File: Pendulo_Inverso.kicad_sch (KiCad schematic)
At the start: 6 parts, among them IC2 TB6612FNG, U1 LM7805_TO220, U2 ESP32-DEVKITC, U4 MPU-6050-A

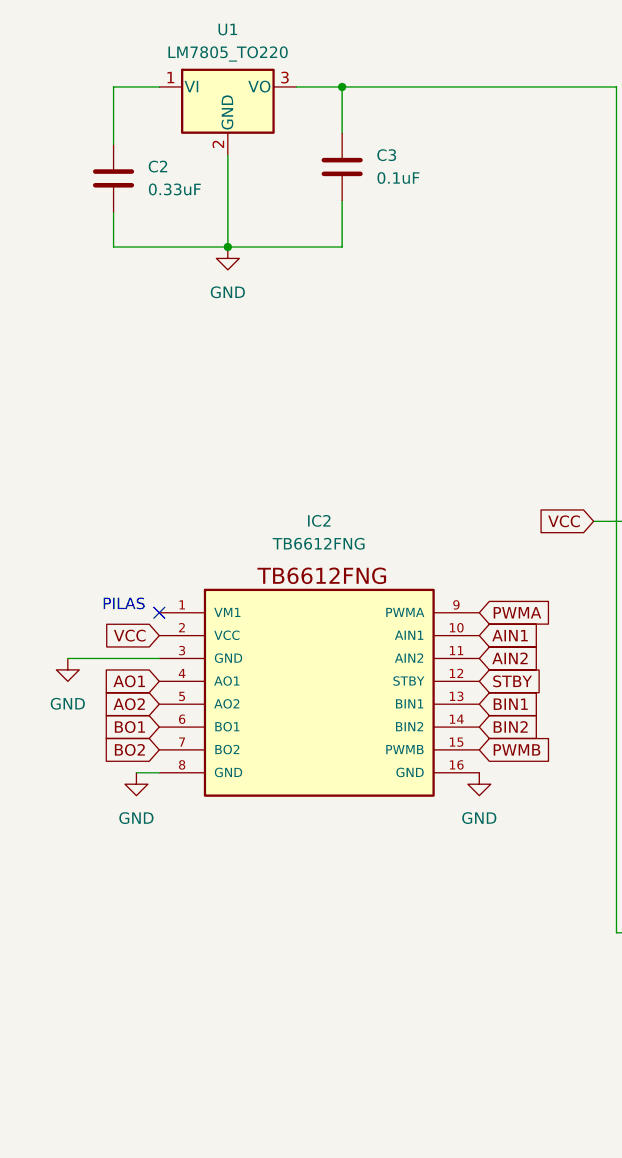
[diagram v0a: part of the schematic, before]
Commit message: modified:   Pendulo_Inverso.dsn 	modified:   Pendulo_Inverso.kicad_pcb 	modified:   Pendulo_Inverso.kicad_prl 	modified:   Pendulo_Inverso.kicad_sch 	modified:   Pendulo_Inverso.rules 	modified:   Pendulo_Inverso.ses 	modified:   fp-info-cache
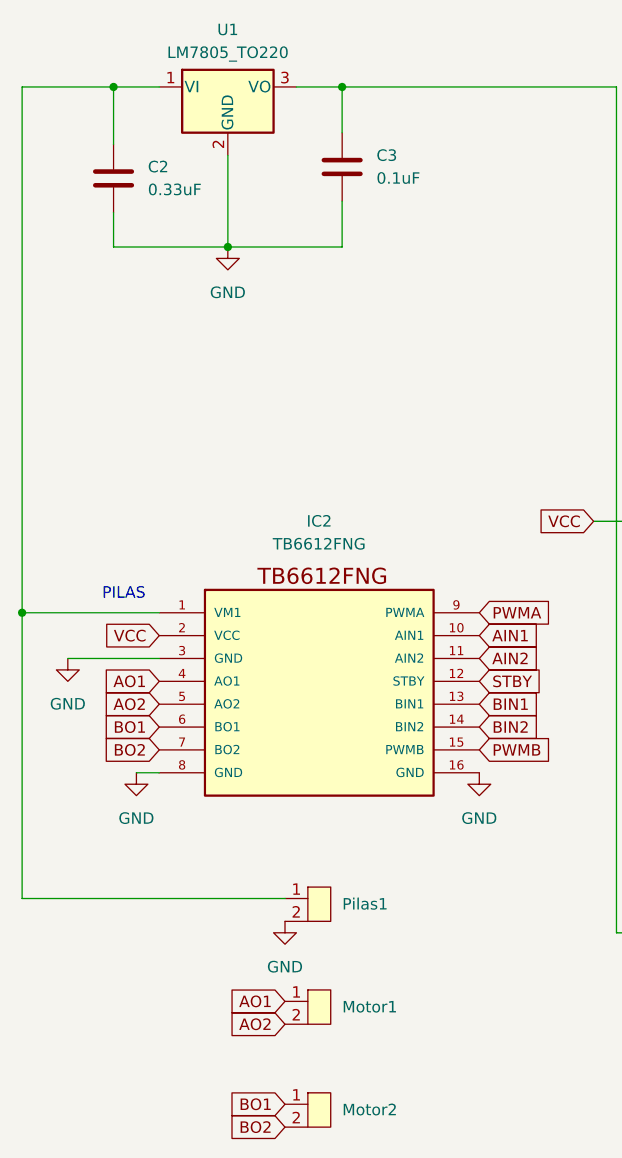
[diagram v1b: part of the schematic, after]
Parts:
- added Motor1, Motor2, Pilas1: ~, Mi_Libreria2:Conector_doble, symbol Mi_Libreria:Conector_doble
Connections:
- net AO1: now also Motor1.1
- net AO2: now also Motor1.2
- net BO1: now also Motor2.1
- net BO2: now also Motor2.2
- net GND: now also Pilas1.2
- net at C2.1, U1.1 (VI): now also IC2.1 (VM1), Pilas1.1
- no-connect marks 31 -> 30
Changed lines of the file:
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@@
   (junction (at 132.08 88.9) (diameter 0) (color 0 0 0 0)
   )
+  (junction (at 60.96 99.06) (diameter 0) (color 0 0 0 0)
+  )
   (junction (at 83.82 58.42) (diameter 0) (color 0 0 0 0)
+  )
+  (junction (at 71.12 40.64) (diameter 0) (color 0 0 0 0)
   )
   (junction (at 96.52 40.64) (diameter 0) (color 0 0 0 0)
@@
   (no_connect (at 132.08 93.98))
   (no_connect (at 132.08 101.6))
-  (no_connect (at 76.2 99.06))
   (no_connect (at 132.08 104.14))
   (no_connect (at 172.72 96.52))
@@
     (stroke (width 0) (type default))
   )
+  (wire (pts (xy 60.96 130.81) (xy 90.17 130.81))
+    (stroke (width 0) (type default))
+  )
   (wire (pts (xy 96.52 40.64) (xy 127 40.64))
     (stroke (width 0) (type default))
@@
     (stroke (width 0) (type default))
   )
+  (wire (pts (xy 71.12 40.64) (xy 60.96 40.64))
+    (stroke (width 0) (type default))
+  )
   (wire (pts (xy 172.72 104.14) (xy 177.8 104.14))
     (stroke (width 0) (type default))
@@
     (stroke (width 0) (type default))
   )
+  (wire (pts (xy 60.96 40.64) (xy 60.96 99.06))
+    (stroke (width 0) (type default))
+  )
   (wire (pts (xy 180.34 101.6) (xy 180.34 104.14))
     (stroke (width 0) (type default))
   )
+  (wire (pts (xy 60.96 99.06) (xy 60.96 130.81))
+    (stroke (width 0) (type default))
+  )
   (wire (pts (xy 71.12 54.61) (xy 71.12 58.42))
     (stroke (width 0) (type default))
@@
     (stroke (width 0) (type default))
   )
+  (wire (pts (xy 76.2 99.06) (xy 60.96 99.06))
+    (stroke (width 0) (type default))
+  )
   (wire (pts (xy 127 134.62) (xy 132.08 134.62))
     (stroke (width 0) (type default))
   )
-  (text "PILAS" (at 69.85 99.06 0)
+  (text "PILAS" (at 69.85 97.79 0)
     (effects (font (size 1.27 1.27)) (justify left bottom))
   )
@@
     )
   )
+  (global_label "AO1" (shape input) (at 90.17 142.24 180) (fields_autoplaced)
+    (effects (font (size 1.27 1.27)) (justify right))
+    (property "Intersheetrefs" "${INTERSHEET_REFS}" (at 83.5562 142.24 0)
+      (effects (font (size 1.27 1.27)) (justify right) hide)
+    )
+  )
   (global_label "BO2" (shape input) (at 76.2 114.3 180) (fields_autoplaced)
     (effects (font (size 1.27 1.27)) (justify right))
@@
     )
   )
+  (global_label "BO2" (shape input) (at 90.17 156.21 180) (fields_autoplaced)
+    (effects (font (size 1.27 1.27)) (justify right))
+    (property "Intersheetrefs" "${INTERSHEET_REFS}" (at 83.3748 156.21 0)
+      (effects (font (size 1.27 1.27)) (justify right) hide)
+    )
+  )
+  (global_label "BO1" (shape input) (at 90.17 153.67 180) (fields_autoplaced)
+    (effects (font (size 1.27 1.27)) (justify right))
+    (property "Intersheetrefs" "${INTERSHEET_REFS}" (at 83.3748 153.67 0)
+      (effects (font (size 1.27 1.27)) (justify right) hide)
+    )
+  )
   (global_label "BIN2" (shape input) (at 111.76 111.76 0) (fields_autoplaced)
     (effects (font (size 1.27 1.27)) (justify left))
@@
     )
   )
+  (global_label "AO2" (shape input) (at 90.17 144.78 180) (fields_autoplaced)
+    (effects (font (size 1.27 1.27)) (justify right))
+    (property "Intersheetrefs" "${INTERSHEET_REFS}" (at 83.5562 144.78 0)
+      (effects (font (size 1.27 1.27)) (justify right) hide)
+    )
+  )
   (global_label "PWMB" (shape input) (at 111.76 114.3 0) (fields_autoplaced)
     (effects (font (size 1.27 1.27)) (justify left))
@@
         (path "/efb3785d-97dd-4c84-bd5b-f8cfd60b2cf2"
           (reference "#PWR04") (unit 1)
+        )
+      )
+    )
+  )
+  (symbol (lib_id "power:GND") (at 90.17 133.35 0) (unit 1)
+    (in_bom yes) (on_board yes) (dnp no) (fields_autoplaced)
+    (property "Reference" "#PWR09" (at 90.17 139.7 0)
+      (effects (font (size 1.27 1.27)) hide)
+    )
+    (property "Value" "GND" (at 90.17 138.43 0)
+      (effects (font (size 1.27 1.27)))
+    )
+    (property "Footprint" "" (at 90.17 133.35 0)
+      (effects (font (size 1.27 1.27)) hide)
+    )
+    (property "Datasheet" "" (at 90.17 133.35 0)
+      (effects (font (size 1.27 1.27)) hide)
+    )
+    (pin "1")
+    (instances
+      (project "Pendulo_Inverso"
+        (path "/efb3785d-97dd-4c84-bd5b-f8cfd60b2cf2"
+          (reference "#PWR09") (unit 1)
+        )
+      )
+    )
+  )
+  (symbol (lib_id "Mi_Libreria:Conector_doble") (at 90.17 153.67 0) (unit 1)
+    (in_bom yes) (on_board yes) (dnp no) (fields_autoplaced)
+    (property "Reference" "Motor2" (at 96.52 154.305 0)
+      (effects (font (size 1.27 1.27)) (justify left))
+    )
+    (property "Value" "~" (at 90.17 153.67 0)
+      (effects (font (size 1.27 1.27)))
+    )
+    (property "Footprint" "Mi_Libreria2:Conector_doble" (at 90.17 153.67 0)
+      (effects (font (size 1.27 1.27)) hide)
+    )
+    (property "Datasheet" "" (at 90.17 153.67 0)
+      (effects (font (size 1.27 1.27)) hide)
+    )
+    (pin "2")
+    (pin "1")
+    (instances
+      (project "Pendulo_Inverso"
+        (path "/efb3785d-97dd-4c84-bd5b-f8cfd60b2cf2"
+          (reference "Motor2") (unit 1)
         )
       )
@@
         (path "/efb3785d-97dd-4c84-bd5b-f8cfd60b2cf2"
           (reference "#PWR08") (unit 1)
+        )
+      )
+    )
+  )
+  (symbol (lib_id "Mi_Libreria:Conector_doble") (at 90.17 130.81 0) (unit 1)
+    (in_bom yes) (on_board yes) (dnp no) (fields_autoplaced)
+    (property "Reference" "Pilas1" (at 96.52 131.445 0)
+      (effects (font (size 1.27 1.27)) (justify left))
+    )
+    (property "Value" "~" (at 90.17 130.81 0)
+      (effects (font (size 1.27 1.27)))
+    )
+    (property "Footprint" "Mi_Libreria2:Conector_doble" (at 90.17 130.81 0)
+      (effects (font (size 1.27 1.27)) hide)
+    )
+    (property "Datasheet" "" (at 90.17 130.81 0)
+      (effects (font (size 1.27 1.27)) hide)
+    )
+    (pin "2")
+    (pin "1")
+    (instances
+      (project "Pendulo_Inverso"
+        (path "/efb3785d-97dd-4c84-bd5b-f8cfd60b2cf2"
+          (reference "Pilas1") (unit 1)
         )
       )
@@
         )
       )
+    )
+  )
+  (symbol (lib_id "Mi_Libreria:Conector_doble") (at 90.17 142.24 0) (unit 1)
+    (in_bom yes) (on_board yes) (dnp no) (fields_autoplaced)
+    (property "Reference" "Motor1" (at 96.52 142.875 0)
+      (effects (font (size 1.27 1.27)) (justify left))
+    )
+    (property "Value" "~" (at 90.17 142.24 0)
+      (effects (font (size 1.27 1.27)))
+    )
+    (property "Footprint" "Mi_Libreria2:Conector_doble" (at 90.17 142.24 0)
+      (effects (font (size 1.27 1.27)) hide)
+    )
+    (property "Datasheet" "" (at 90.17 142.24 0)
+      (effects (font (size 1.27 1.27)) hide)
+    )
+    (pin "2")
+    (pin "1")
+    (instances
+      (project "Pendulo_Inverso"
+        (path "/efb3785d-97dd-4c84-bd5b-f8cfd60b2cf2"
+          (reference "Motor1") (unit 1)
+        )
+      )

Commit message: new file:   Pendulo_Inverso-backups/Pendulo_Inverso-2024-04-04_134628.zip 	modified:   Pendulo_Inverso.kicad_pcb 	modified:   Pendulo_Inverso.kicad_prl 	modified:   Pendulo_Inverso.kicad_pro 	modified:   Pendulo_Inverso.kicad_sch 	modified:   fp-info-cache
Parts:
- C2, C3: footprint Capacitor_SMD:CP_Elec_3x5.3 -> Capacitor_THT:CP_Radial_D8.0mm_P3.50mm
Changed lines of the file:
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@@
       (effects (font (size 1.27 1.27)) (justify left))
     )
-    (property "Footprint" "Capacitor_SMD:CP_Elec_3x5.3" (at 72.0852 54.61 0)
+    (property "Footprint" "Capacitor_THT:CP_Radial_D8.0mm_P3.50mm" (at 72.0852 54.61 0)
       (effects (font (size 1.27 1.27)) hide)
     )
@@
       (effects (font (size 1.27 1.27)) (justify left))
     )
-    (property "Footprint" "Capacitor_SMD:CP_Elec_3x5.3" (at 97.4852 53.34 0)
-      (effects (font (size 1.27 1.27)) hide)
-    )
+    (property "Footprint" "Capacitor_THT:CP_Radial_D8.0mm_P3.50mm" (at 97.4852 53.34 0)
+      (effects (font (size 1.27 1.27)) hide)
+    )

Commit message: deleted:    Pendulo_Inverso-backups/Pendulo_Inverso-2024-03-22_111232.zip 	new file:   Pendulo_Inverso-backups/Pendulo_Inverso-2024-04-06_125540.zip 	new file:   Pendulo_Inverso-backups/Pendulo_Inverso-2024-04-11_225156.zip 	new file:   Pendulo_Inverso-backups/Pendulo_Inverso-2024-04-11_230001.zip 	new file:   Pendulo_Inverso-backups/Pendulo_Inverso-2024-04-11_230555.zip 	modified:   Pendulo_Inverso.kicad_pcb 	modified:   Pendulo_Inverso.kicad_prl 	modified:   Pendulo_Inverso.kicad_sch
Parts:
- Motor1, Motor2, Pilas1: footprint Mi_Libreria2:Conector_doble -> TerminalBlock_Phoenix:TerminalBlock_Phoenix_MKDS-1,5-2_1x02_P5.00mm_Horizontal
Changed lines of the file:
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@@
       (effects (font (size 1.27 1.27)))
     )
-    (property "Footprint" "Mi_Libreria2:Conector_doble" (at 90.17 153.67 0)
+    (property "Footprint" "TerminalBlock_Phoenix:TerminalBlock_Phoenix_MKDS-1,5-2_1x02_P5.00mm_Horizontal" (at 90.17 153.67 0)
       (effects (font (size 1.27 1.27)) hide)
     )
@@
       (effects (font (size 1.27 1.27)))
     )
-    (property "Footprint" "Mi_Libreria2:Conector_doble" (at 90.17 130.81 0)
+    (property "Footprint" "TerminalBlock_Phoenix:TerminalBlock_Phoenix_MKDS-1,5-2_1x02_P5.00mm_Horizontal" (at 90.17 130.81 0)
       (effects (font (size 1.27 1.27)) hide)
     )
@@
       (effects (font (size 1.27 1.27)))
     )
-    (property "Footprint" "Mi_Libreria2:Conector_doble" (at 90.17 142.24 0)
-      (effects (font (size 1.27 1.27)) hide)
-    )
+    (property "Footprint" "TerminalBlock_Phoenix:TerminalBlock_Phoenix_MKDS-1,5-2_1x02_P5.00mm_Horizontal" (at 90.17 142.24 0)
+      (effects (font (size 1.27 1.27)) hide)
+    )
